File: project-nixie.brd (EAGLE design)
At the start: 22.5 x 29.2 mm, 8 parts, among them J1 D

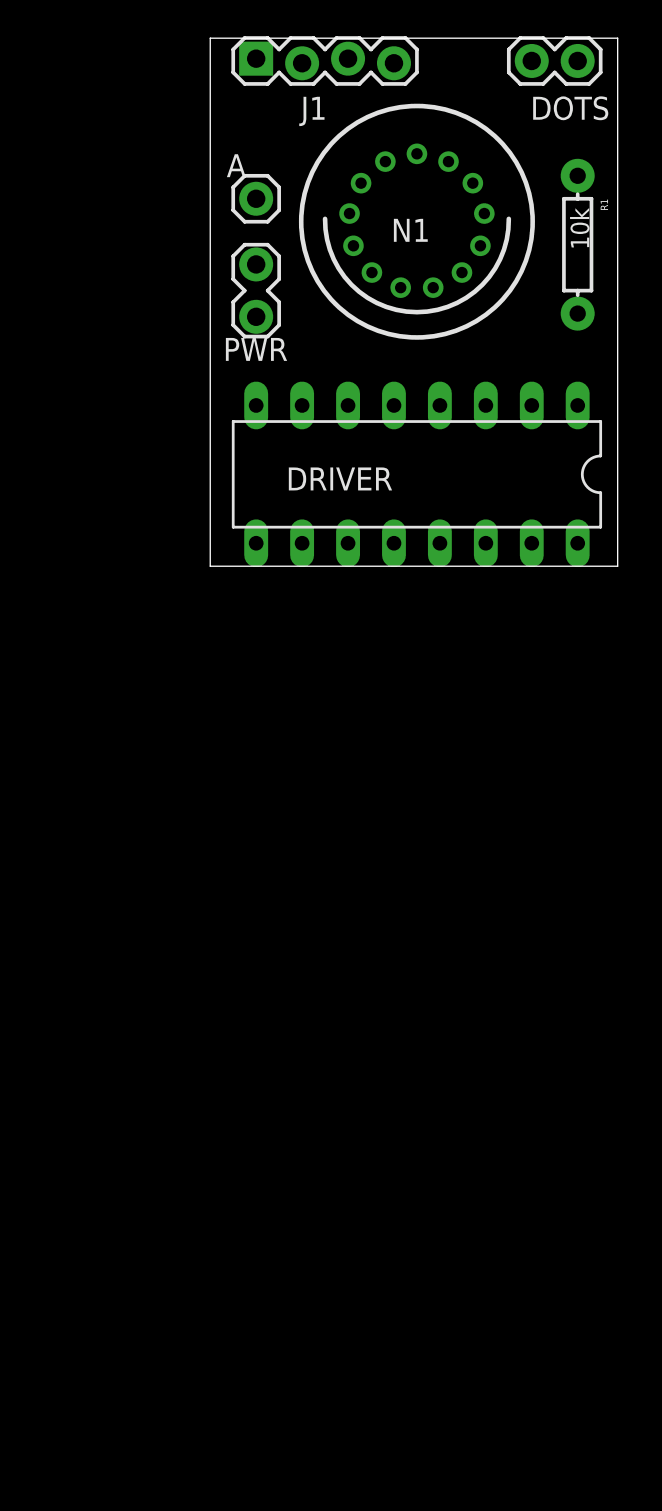
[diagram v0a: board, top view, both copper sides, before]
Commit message: re-upload to seeed
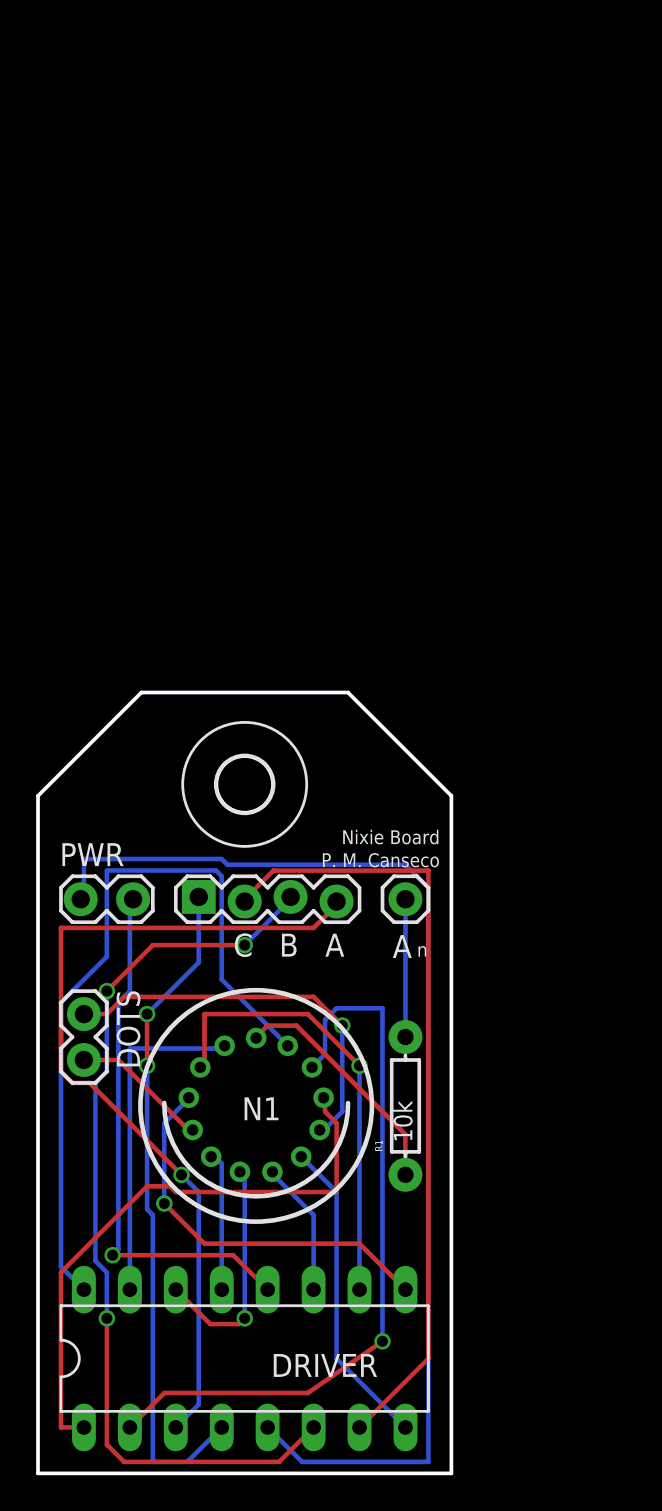
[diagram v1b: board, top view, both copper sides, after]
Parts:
- removed FRAME1: FRAME-LETTER, SparkFun-Aesthetics:CREATIVE_COMMONS
- added U$1: (no value), holes:3,0
- moved DOTS 58.2 mm to (1.91, 24.8), turned to 270 degrees
- moved DRIVER 49.8 mm to (10.8, 5.71), turned to 0 degrees
- moved N1 49.7 mm to (11.4, 19.7)
- moved R1 48.6 mm to (19.7, 19.7), turned to 90 degrees
- moved J1 46.5 mm to (8.26, 31.1)
- moved A 39.6 mm to (19.7, 31.1), turned to 0 degrees
- moved PWR 33.8 mm to (1.91, 31.1), turned to 0 degrees
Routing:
- net 5V: track 0.00 -> 63.5 mm
- net B: track 0.00 -> 50.6 mm, vias 0 -> 3
- net A: track 0.00 -> 47.8 mm, vias 0 -> 1
- net C: track 0.00 -> 43.3 mm
- net N$10: track 0.00 -> 42.1 mm
- net N$1: track 0.00 -> 40.4 mm, vias 0 -> 1
- net D: track 0.00 -> 37.2 mm, vias 0 -> 2
- net N$2: track 0.00 -> 32.7 mm
- net GND: track 0.00 -> 29.6 mm, vias 0 -> 1
- net N$3: track 0.00 -> 25.2 mm, vias 0 -> 1
- net LHDP: track 0.00 -> 21.8 mm, vias 0 -> 1
- net N$7: track 0.00 -> 21.7 mm, vias 0 -> 1
- net N$9: track 0.00 -> 18.6 mm
- net N$8: track 0.00 -> 17.4 mm
- net N$11: track 0.00 -> 13.3 mm
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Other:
- board size 22.5 x 29.2 mm -> 22.9 x 43.2 mm
- board text added: "A"
- board text added: "B"
- board text added: "C"
- board text added: "Nixie Board"
- board text added: "P. M. Canseco"
- board text added: "n"
